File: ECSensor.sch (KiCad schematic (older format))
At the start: 8 parts, among them J2 EC_Sensor_Input_3_Pin, Q2 Q_PMOS_DSG

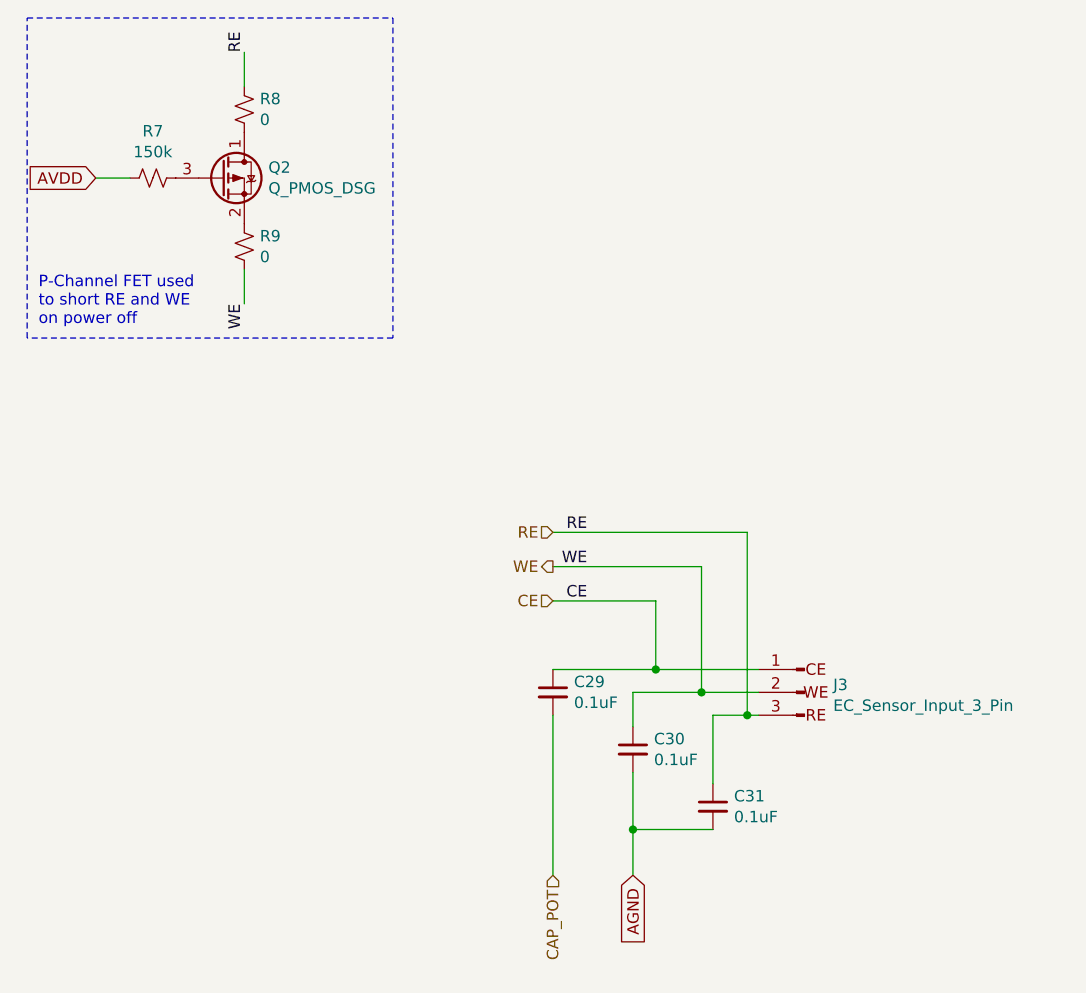
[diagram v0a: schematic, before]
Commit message: beginning layout
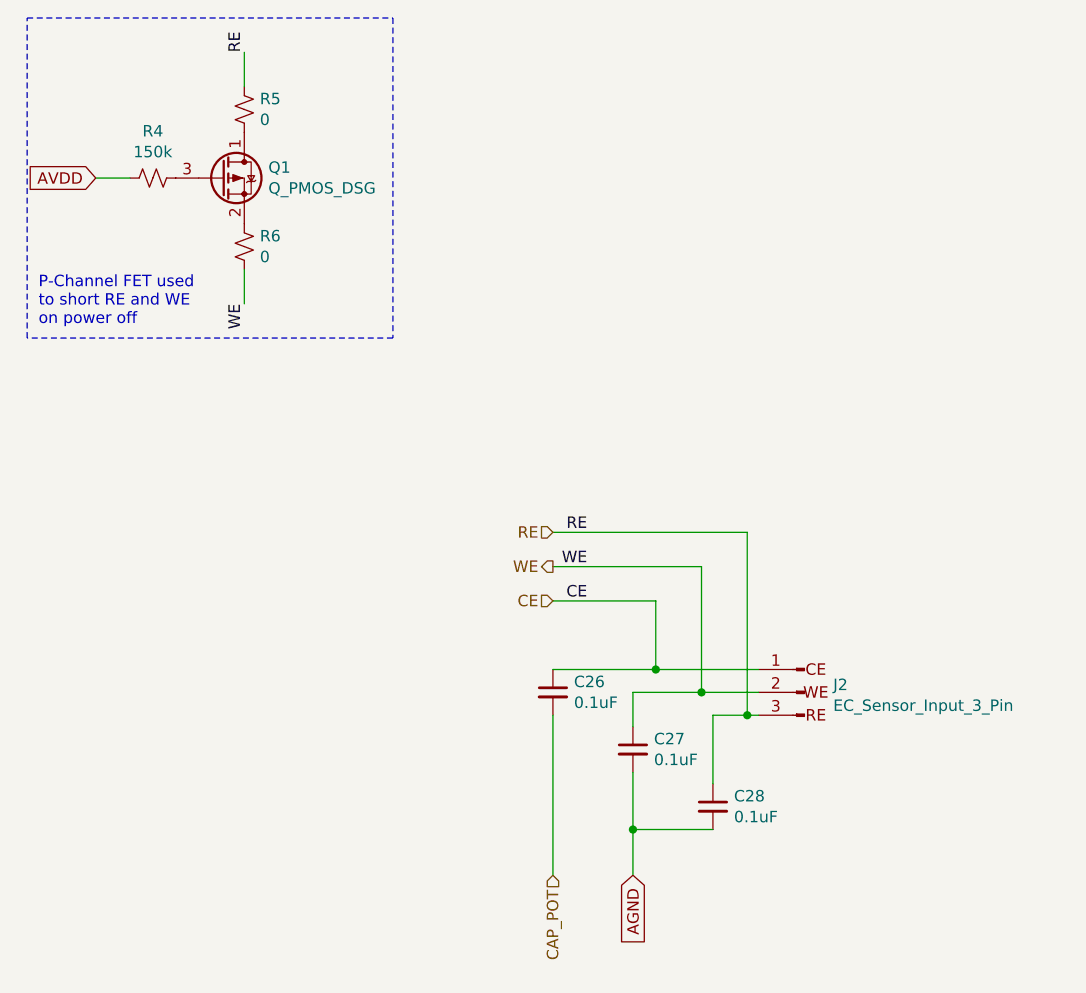
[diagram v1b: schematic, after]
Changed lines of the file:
@@
 EESchema Schematic File Version 4
+LIBS:aducm_board-cache
 EELAYER 30 0
 EELAYER END
 $Descr A4 11693 8268
 encoding utf-8
-Sheet 3 5
+Sheet 2 5
 Title "ADuCM355 Template"
 Date ""
@@
 AR Path="/5DF7340A/5DF76279" Ref="C27"  Part="1"
 AR Path="/5DF54D0C/5DF76279" Ref="C30"  Part="1"
-F 0 "C30" H 3442 3896 50  0000 L CNN
+F 0 "C27" H 3442 3896 50  0000 L CNN
 F 1 "0.1uF" H 3442 3805 50  0000 L CNN
 F 2 "Capacitor_SMD:C_0603_1608Metric" H 3350 3850 50  0001 C CNN
@@
 AR Path="/5DF7340A/5DF76497" Ref="C26"  Part="1"
 AR Path="/5DF54D0C/5DF76497" Ref="C29"  Part="1"
-F 0 "C29" H 3092 3646 50  0000 L CNN
+F 0 "C26" H 3092 3646 50  0000 L CNN
 F 1 "0.1uF" H 3092 3555 50  0000 L CNN
 F 2 "Capacitor_SMD:C_0603_1608Metric" H 3000 3600 50  0001 C CNN
@@
 AR Path="/5DF7340A/5DF768A0" Ref="C28"  Part="1"
 AR Path="/5DF54D0C/5DF768A0" Ref="C31"  Part="1"
-F 0 "C31" H 3792 4146 50  0000 L CNN
+F 0 "C28" H 3792 4146 50  0000 L CNN
 F 1 "0.1uF" H 3792 4055 50  0000 L CNN
 F 2 "Capacitor_SMD:C_0603_1608Metric" H 3700 4100 50  0001 C CNN
@@
 AR Path="/5DF7340A/5DF7EEA4" Ref="J2"  Part="1"
 AR Path="/5DF54D0C/5DF7EEA4" Ref="J3"  Part="1"
-F 0 "J3" H 3974 3633 50  0000 R CNN
+F 0 "J2" H 3974 3633 50  0000 R CNN
 F 1 "EC_Sensor_Input_3_Pin" H 3974 3542 50  0000 R CNN
 F 2 "Connector_PinHeader_2.54mm:PinHeader_1x03_P2.54mm_Horizontal" H 4100 3600 50  0001 C CNN
@@
 AR Path="/5DF54D0C/5E0080C3" Ref="Q2"  Part="1"
 AR Path="/5DF7340A/5E0080C3" Ref="Q1"  Part="1"
-F 0 "Q2" H 1755 1396 50  0000 L CNN
+F 0 "Q1" H 1755 1396 50  0000 L CNN
 F 1 "Q_PMOS_DSG" H 1755 1305 50  0000 L CNN
 F 2 "Package_TO_SOT_SMD:SOT-23" H 1750 1450 50  0001 C CNN
@@
 AR Path="/5DF54D0C/5E00BDC0" Ref="R7"  Part="1"
 AR Path="/5DF7340A/5E00BDC0" Ref="R4"  Part="1"
-F 0 "R7" V 1045 1350 50  0000 C CNN
+F 0 "R4" V 1045 1350 50  0000 C CNN
 F 1 "150k" V 1136 1350 50  0000 C CNN
 F 2 "Resistor_SMD:R_0603_1608Metric" H 1250 1350 50  0001 C CNN
@@
 AR Path="/5DF54D0C/5E00C4B8" Ref="R8"  Part="1"
 AR Path="/5DF7340A/5E00C4B8" Ref="R5"  Part="1"
-F 0 "R8" H 1582 1004 50  0000 R CNN
+F 0 "R5" H 1582 1004 50  0000 R CNN
 F 1 "0" H 1582 1095 50  0000 R CNN
 F 2 "Resistor_SMD:R_0603_1608Metric" H 1650 1050 50  0001 C CNN
@@
 AR Path="/5DF54D0C/5E00C73E" Ref="R9"  Part="1"
 AR Path="/5DF7340A/5E00C73E" Ref="R6"  Part="1"
-F 0 "R9" H 1718 1696 50  0000 L CNN
+F 0 "R6" H 1718 1696 50  0000 L CNN
 F 1 "0" H 1718 1605 50  0000 L CNN
 F 2 "Resistor_SMD:R_0603_1608Metric" H 1650 1650 50  0001 C CNN

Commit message: io layout finished
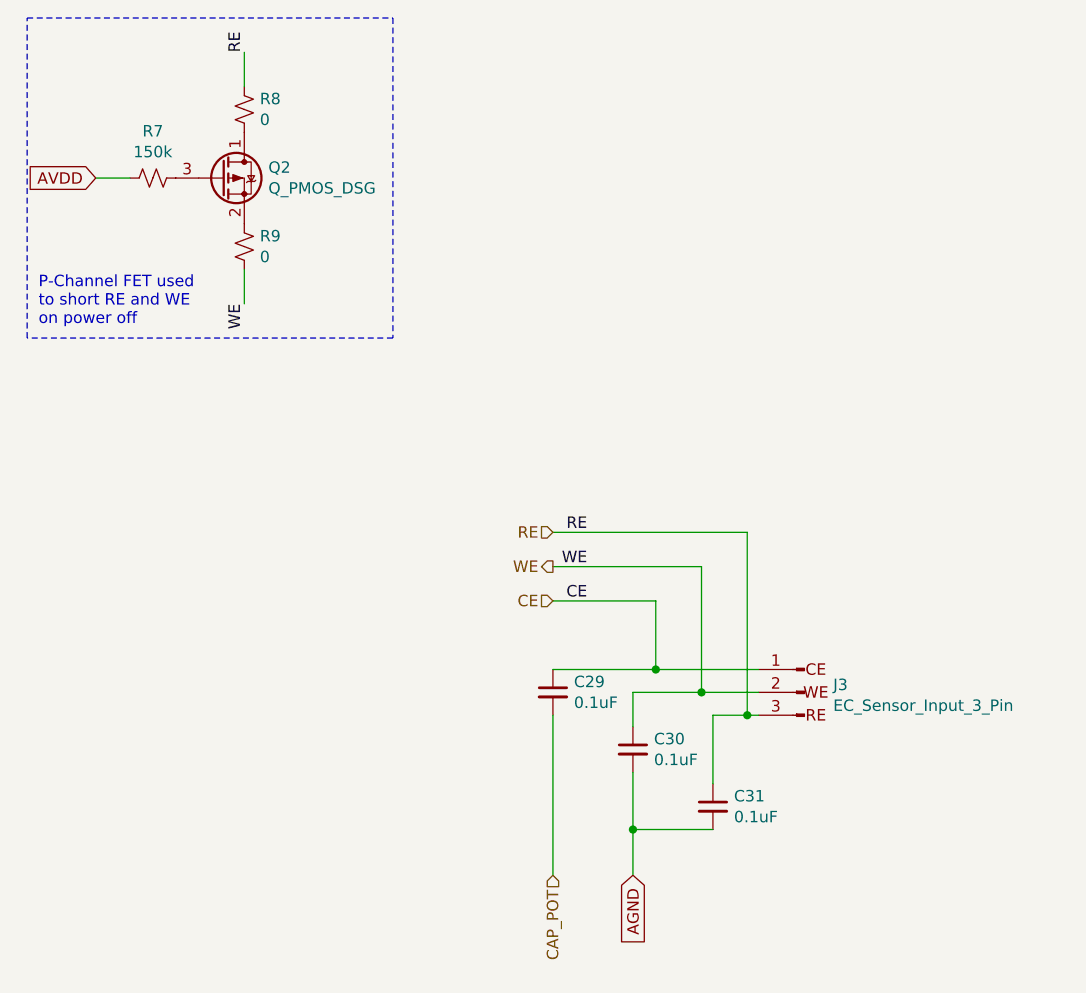
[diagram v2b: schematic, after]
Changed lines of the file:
@@
 $Descr A4 11693 8268
 encoding utf-8
-Sheet 2 5
+Sheet 3 5
 Title "ADuCM355 Template"
 Date ""
@@
 AR Path="/5DF7340A/5DF76279" Ref="C27"  Part="1"
 AR Path="/5DF54D0C/5DF76279" Ref="C30"  Part="1"
-F 0 "C27" H 3442 3896 50  0000 L CNN
+F 0 "C30" H 3442 3896 50  0000 L CNN
 F 1 "0.1uF" H 3442 3805 50  0000 L CNN
 F 2 "Capacitor_SMD:C_0603_1608Metric" H 3350 3850 50  0001 C CNN
@@
 AR Path="/5DF7340A/5DF76497" Ref="C26"  Part="1"
 AR Path="/5DF54D0C/5DF76497" Ref="C29"  Part="1"
-F 0 "C26" H 3092 3646 50  0000 L CNN
+F 0 "C29" H 3092 3646 50  0000 L CNN
 F 1 "0.1uF" H 3092 3555 50  0000 L CNN
 F 2 "Capacitor_SMD:C_0603_1608Metric" H 3000 3600 50  0001 C CNN
@@
 AR Path="/5DF7340A/5DF768A0" Ref="C28"  Part="1"
 AR Path="/5DF54D0C/5DF768A0" Ref="C31"  Part="1"
-F 0 "C28" H 3792 4146 50  0000 L CNN
+F 0 "C31" H 3792 4146 50  0000 L CNN
 F 1 "0.1uF" H 3792 4055 50  0000 L CNN
 F 2 "Capacitor_SMD:C_0603_1608Metric" H 3700 4100 50  0001 C CNN
@@
 AR Path="/5DF7340A/5DF7EEA4" Ref="J2"  Part="1"
 AR Path="/5DF54D0C/5DF7EEA4" Ref="J3"  Part="1"
-F 0 "J2" H 3974 3633 50  0000 R CNN
+F 0 "J3" H 3974 3633 50  0000 R CNN
 F 1 "EC_Sensor_Input_3_Pin" H 3974 3542 50  0000 R CNN
 F 2 "Connector_PinHeader_2.54mm:PinHeader_1x03_P2.54mm_Horizontal" H 4100 3600 50  0001 C CNN
@@
 AR Path="/5DF54D0C/5E0080C3" Ref="Q2"  Part="1"
 AR Path="/5DF7340A/5E0080C3" Ref="Q1"  Part="1"
-F 0 "Q1" H 1755 1396 50  0000 L CNN
+F 0 "Q2" H 1755 1396 50  0000 L CNN
 F 1 "Q_PMOS_DSG" H 1755 1305 50  0000 L CNN
 F 2 "Package_TO_SOT_SMD:SOT-23" H 1750 1450 50  0001 C CNN
@@
 AR Path="/5DF54D0C/5E00BDC0" Ref="R7"  Part="1"
 AR Path="/5DF7340A/5E00BDC0" Ref="R4"  Part="1"
-F 0 "R4" V 1045 1350 50  0000 C CNN
+F 0 "R7" V 1045 1350 50  0000 C CNN
 F 1 "150k" V 1136 1350 50  0000 C CNN
 F 2 "Resistor_SMD:R_0603_1608Metric" H 1250 1350 50  0001 C CNN
@@
 AR Path="/5DF54D0C/5E00C4B8" Ref="R8"  Part="1"
 AR Path="/5DF7340A/5E00C4B8" Ref="R5"  Part="1"
-F 0 "R5" H 1582 1004 50  0000 R CNN
+F 0 "R8" H 1582 1004 50  0000 R CNN
 F 1 "0" H 1582 1095 50  0000 R CNN
 F 2 "Resistor_SMD:R_0603_1608Metric" H 1650 1050 50  0001 C CNN
@@
 AR Path="/5DF54D0C/5E00C73E" Ref="R9"  Part="1"
 AR Path="/5DF7340A/5E00C73E" Ref="R6"  Part="1"
-F 0 "R6" H 1718 1696 50  0000 L CNN
+F 0 "R9" H 1718 1696 50  0000 L CNN
 F 1 "0" H 1718 1605 50  0000 L CNN
 F 2 "Resistor_SMD:R_0603_1608Metric" H 1650 1650 50  0001 C CNN
